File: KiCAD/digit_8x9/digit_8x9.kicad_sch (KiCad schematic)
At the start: 3 parts, among them U1 4514, U2 74HC595

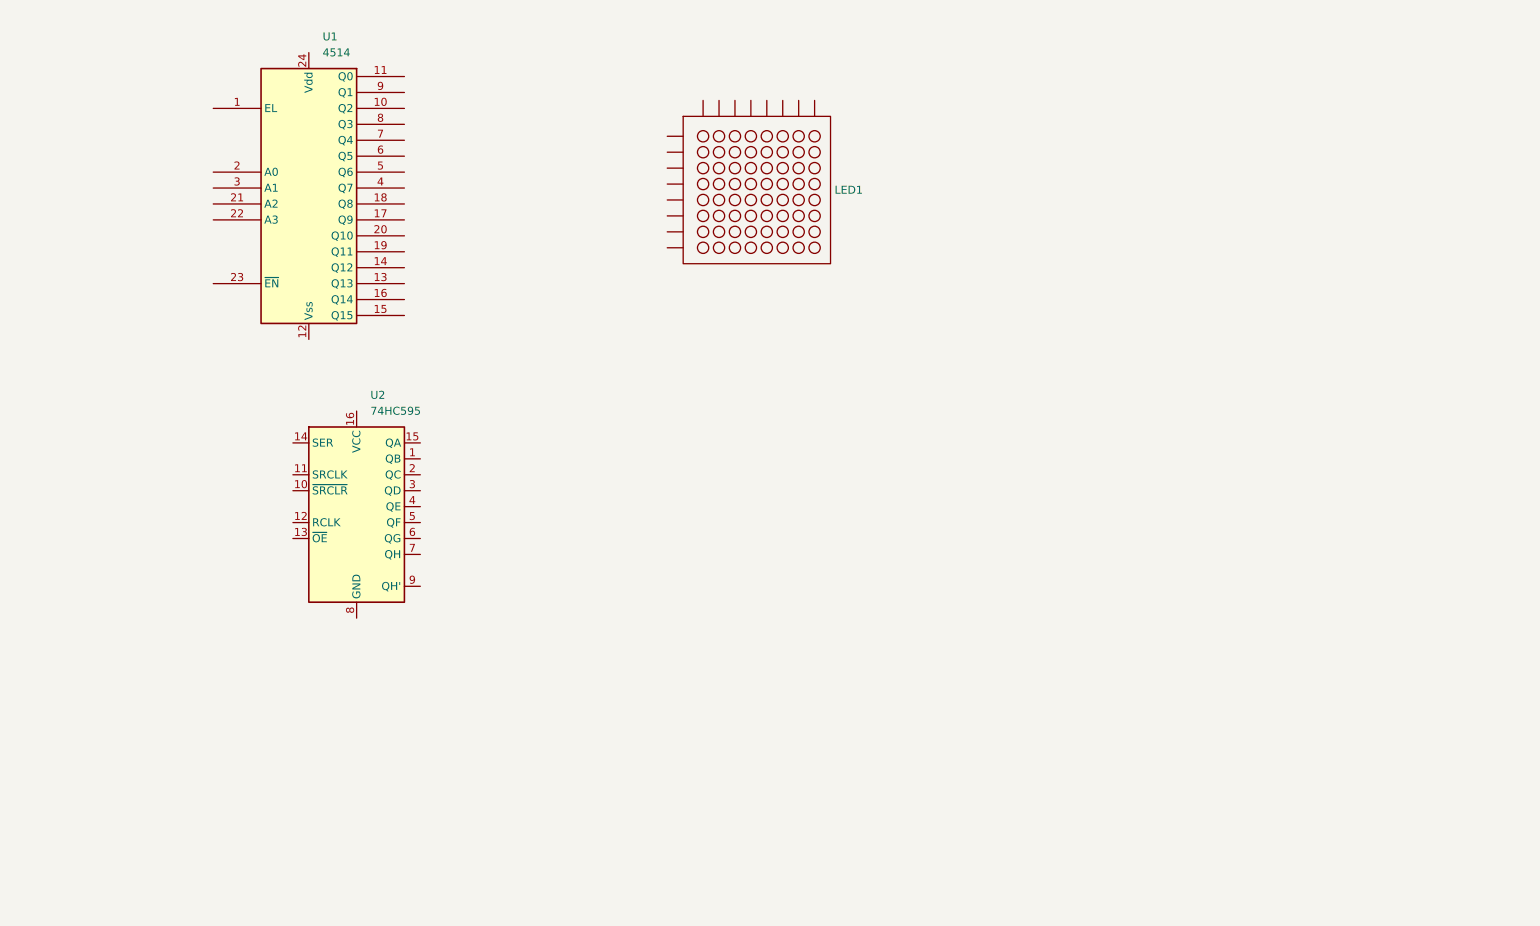
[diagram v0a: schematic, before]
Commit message: schematic work
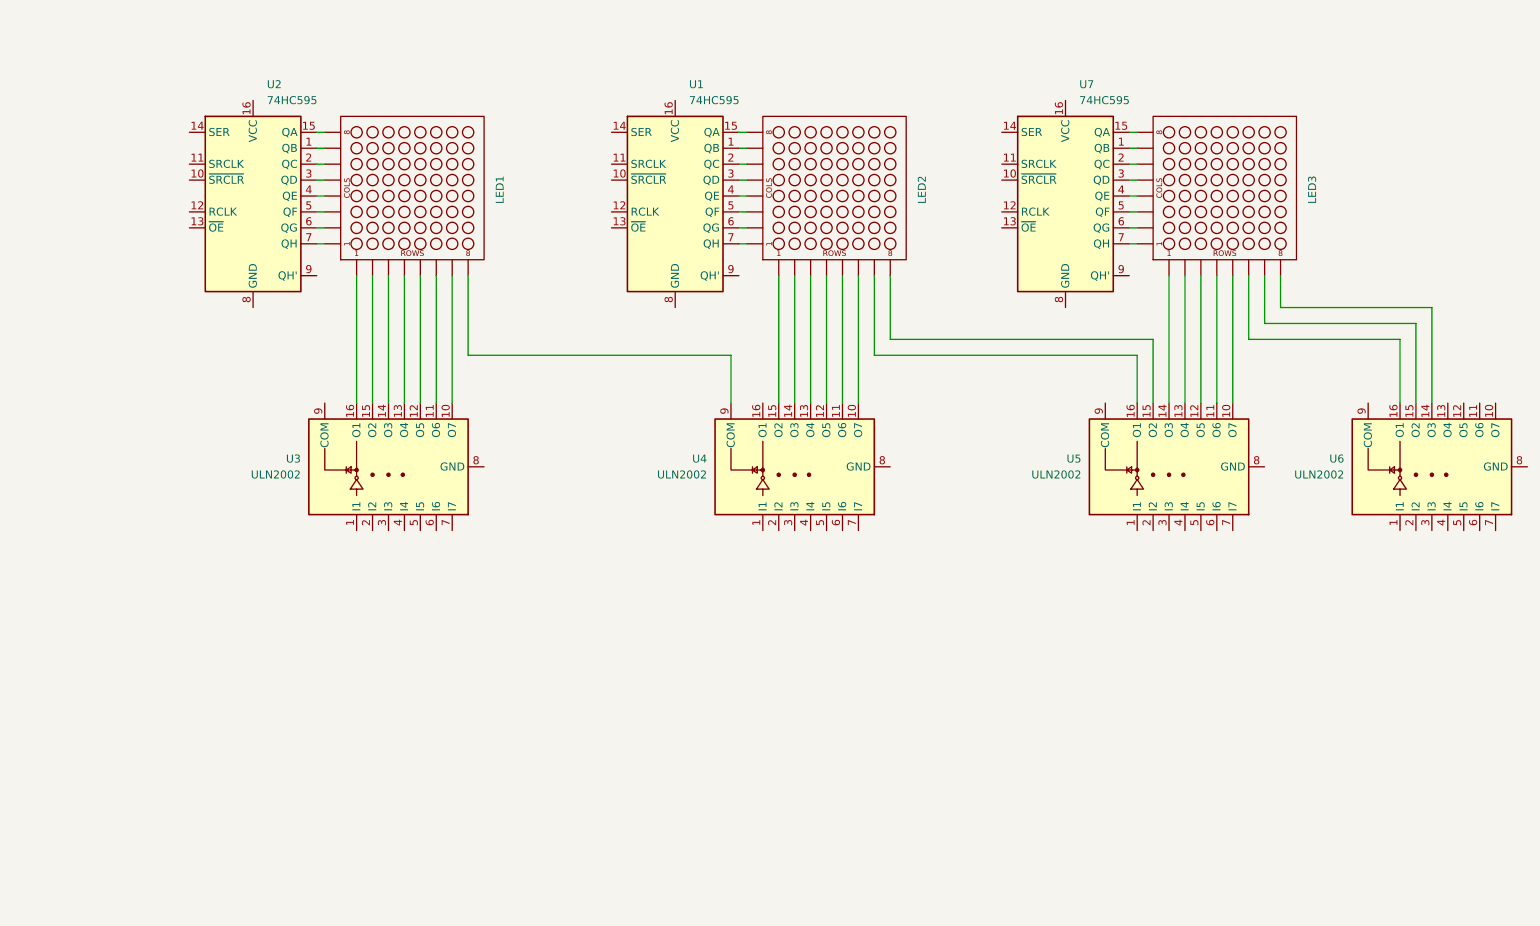
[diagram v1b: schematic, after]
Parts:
- removed U1: 4514, symbol 4xxx_IEEE:4514
- added LED2, LED3: ~, symbol my_led:adafruit_8x8_cc
- added U1, U7: 74HC595, symbol 74xx:74HC595
- added U3, U4, U5, U6: ULN2002, symbol Transistor_Array:ULN2002
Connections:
- net at U2.1 (QB): now also LED1.15 (COL7)
- net at U2.15 (QA): now also LED1.16 (COL8)
- net at U2.2 (QC): now also LED1.11 (COL6)
- net at U2.3 (QD): now also LED1.6 (COL5)
- net at U2.4 (QE): now also LED1.10 (COL4)
- net at U2.5 (QF): now also LED1.4 (COL3)
- net at U2.6 (QG): now also LED1.3 (COL2)
- net at U2.7 (QH): now also LED1.13 (COL1)
- net at LED1.1 (ROW5): now also U3.12 (O5)
- net at LED1.12 (ROW4): now also U3.13 (O4)
- net at LED1.14 (ROW2): now also U3.15 (O2)
- net at LED1.2 (ROW7): now also U3.10 (O7)
- net at LED1.5 (ROW8): now also U4.9 (COM)
- net at LED1.7 (ROW6): now also U3.11 (O6)
- net at LED1.8 (ROW3): now also U3.14 (O3)
- net at LED1.9 (ROW1): now also U3.16 (O1)
- new net: LED3.1 (ROW5), U5.10 (O7)
- new net: LED3.10 (COL4), U7.4 (QE)
- new net: LED3.11 (COL6), U7.2 (QC)
- new net: LED3.12 (ROW4), U5.11 (O6)
- new net: LED3.13 (COL1), U7.7 (QH)
- new net: LED3.14 (ROW2), U5.13 (O4)
- new net: LED3.15 (COL7), U7.1 (QB)
- new net: LED3.16 (COL8), U7.15 (QA)
- new net: LED3.2 (ROW7), U6.15 (O2)
- new net: LED3.3 (COL2), U7.6 (QG)
- new net: LED3.4 (COL3), U7.5 (QF)
- new net: LED3.5 (ROW8), U6.14 (O3)
- new net: LED3.6 (COL5), U7.3 (QD)
- new net: LED3.7 (ROW6), U6.16 (O1)
- new net: LED3.8 (ROW3), U5.12 (O5)
- new net: LED3.9 (ROW1), U5.14 (O3)
- new net: LED2.15 (COL7), U1.1 (QB)
- new net: LED2.16 (COL8), U1.15 (QA)
- new net: LED2.11 (COL6), U1.2 (QC)
- new net: LED2.6 (COL5), U1.3 (QD)
- new net: LED2.10 (COL4), U1.4 (QE)
- new net: LED2.4 (COL3), U1.5 (QF)
- new net: LED2.3 (COL2), U1.6 (QG)
- new net: LED2.13 (COL1), U1.7 (QH)
- new net: LED2.1 (ROW5), U4.11 (O6)
- new net: LED2.12 (ROW4), U4.12 (O5)
- new net: LED2.14 (ROW2), U4.14 (O3)
- new net: LED2.2 (ROW7), U5.16 (O1)
- new net: LED2.5 (ROW8), U5.15 (O2)
- new net: LED2.7 (ROW6), U4.10 (O7)
- new net: LED2.8 (ROW3), U4.13 (O4)
- new net: LED2.9 (ROW1), U4.15 (O2)
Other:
- moved on the sheet: U2

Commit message: Atmega version
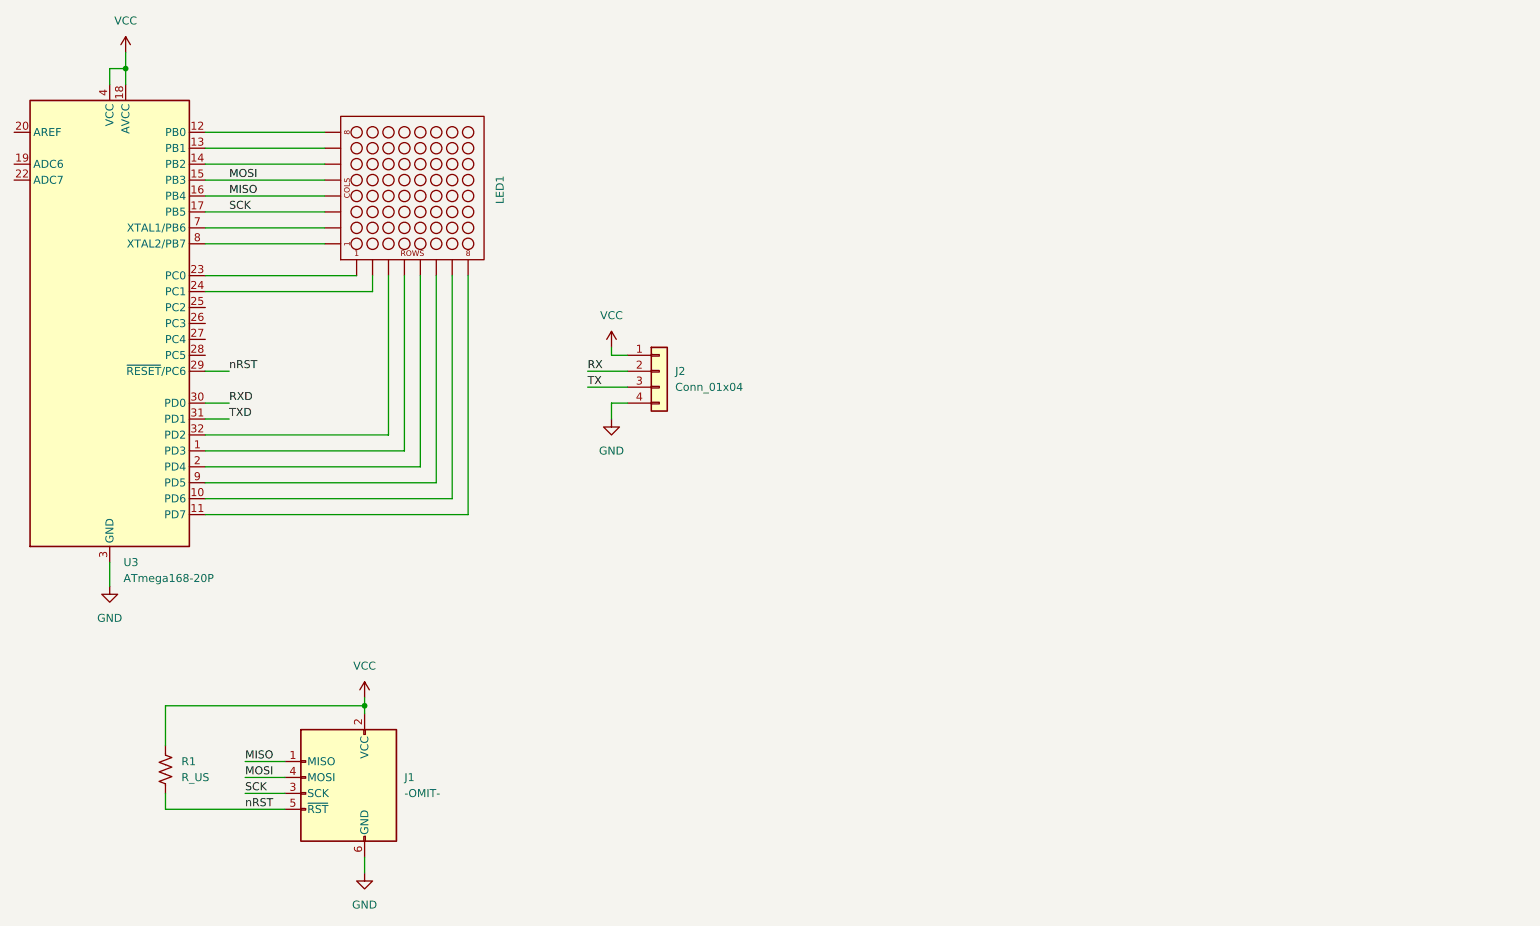
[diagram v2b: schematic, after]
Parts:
- removed LED2, LED3: ~, symbol my_led:adafruit_8x8_cc
- removed U1, U2, U7: 74HC595, symbol 74xx:74HC595
- removed U3, U4, U5, U6: ULN2002, symbol Transistor_Array:ULN2002
- added J1: -OMIT-, Connector_PinHeader_2.54mm:PinHeader_2x03_P2.54mm_Vertical, symbol Connector:AVR-ISP-6
- added J2: Conn_01x04, Connector_PinHeader_2.54mm:PinHeader_1x04_P2.54mm_Vertical, symbol Connector_Generic:Conn_01x04
- added R1: R_US, Resistor_SMD:R_0805_2012Metric_Pad1.20x1.40mm_HandSolder, symbol Device:R_US
- added U3: ATmega168-20P, Package_QFP:TQFP-32_7x7mm_P0.8mm, symbol MCU_Microchip_ATmega:ATmega168A-A
- LED1: footprint (none) -> my_led_array:Adafruit_32mm_8x8
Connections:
- net at LED1.15 (COL7): now also U3.13 (PB1)
- net at LED1.16 (COL8): now also U3.12 (PB0)
- net at LED1.11 (COL6): now also U3.14 (PB2)
- net MOSI: now reaches LED1.6 (COL5)
- net MOSI: now also J1.4 (MOSI), U3.15 (PB3)
- net MISO: now reaches LED1.10 (COL4)
- net MISO: now also J1.1 (MISO), U3.16 (PB4)
- net SCK: now reaches LED1.4 (COL3)
- net SCK: now also J1.3 (SCK), U3.17 (PB5)
- net at LED1.3 (COL2): now also U3.7 (XTAL1/PB6)
- net at LED1.13 (COL1): now also U3.8 (XTAL2/PB7)
- net at LED1.2 (ROW7): now also U3.10 (PD6)
- net at LED1.7 (ROW6): now also U3.9 (PD5)
- net at LED1.1 (ROW5): now also U3.2 (PD4)
- net at LED1.12 (ROW4): now also U3.1 (PD3)
- net at LED1.8 (ROW3): now also U3.32 (PD2)
- net at LED1.14 (ROW2): now also U3.24 (PC1)
- net at LED1.9 (ROW1): now also U3.23 (PC0)
- net at LED1.5 (ROW8): now also U3.11 (PD7)
- new net GND: J1.6 (GND), J2.4 (Pin_4), U3.21 (GND), U3.3 (GND), U3.5 (GND)
- new net RX: J2.2 (Pin_2)
- new net RXD: U3.30 (PD0)
- new net TX: J2.3 (Pin_3)
- new net TXD: U3.31 (PD1)
- new net VCC: J1.2 (VCC), J2.1 (Pin_1), R1.1, U3.18 (AVCC), U3.4 (VCC), U3.6 (VCC)
- new net nRST: J1.5 (~{RST}), R1.2, U3.29 (~{RESET}/PC6)
